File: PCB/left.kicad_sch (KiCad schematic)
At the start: 3 parts, among them J1 AudioJack4, U1 MOUDLE-SEEEDUINO-XIAO, U2 MCP23017_ML

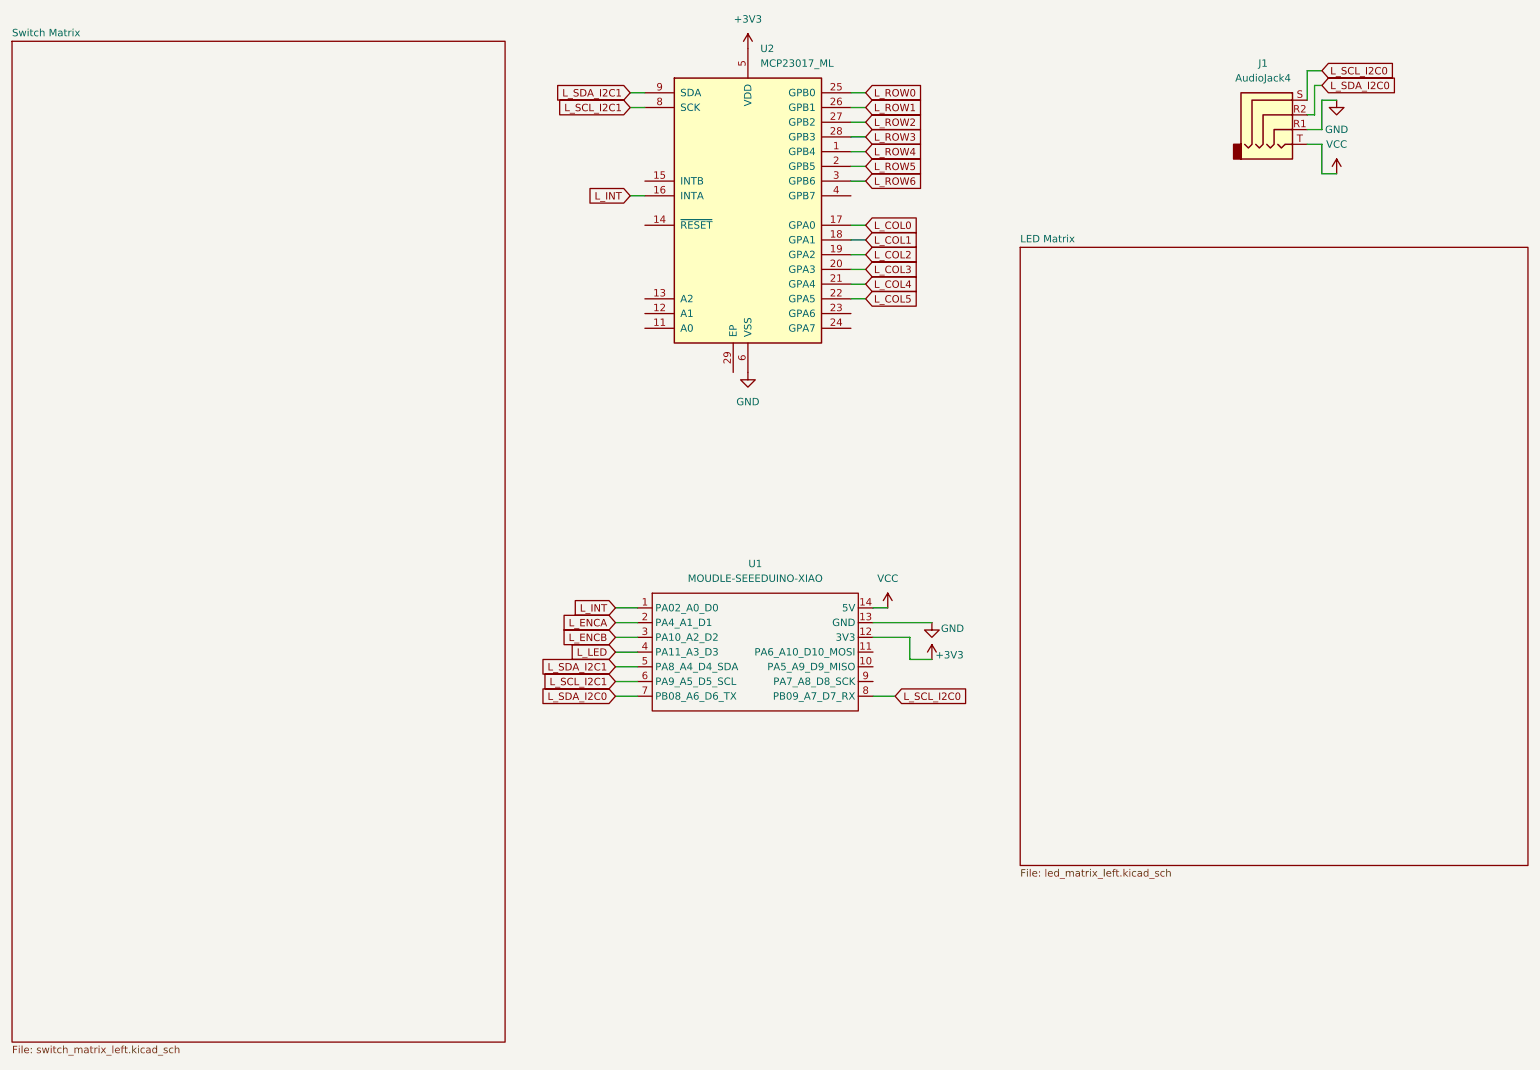
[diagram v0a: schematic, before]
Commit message: updated schematic
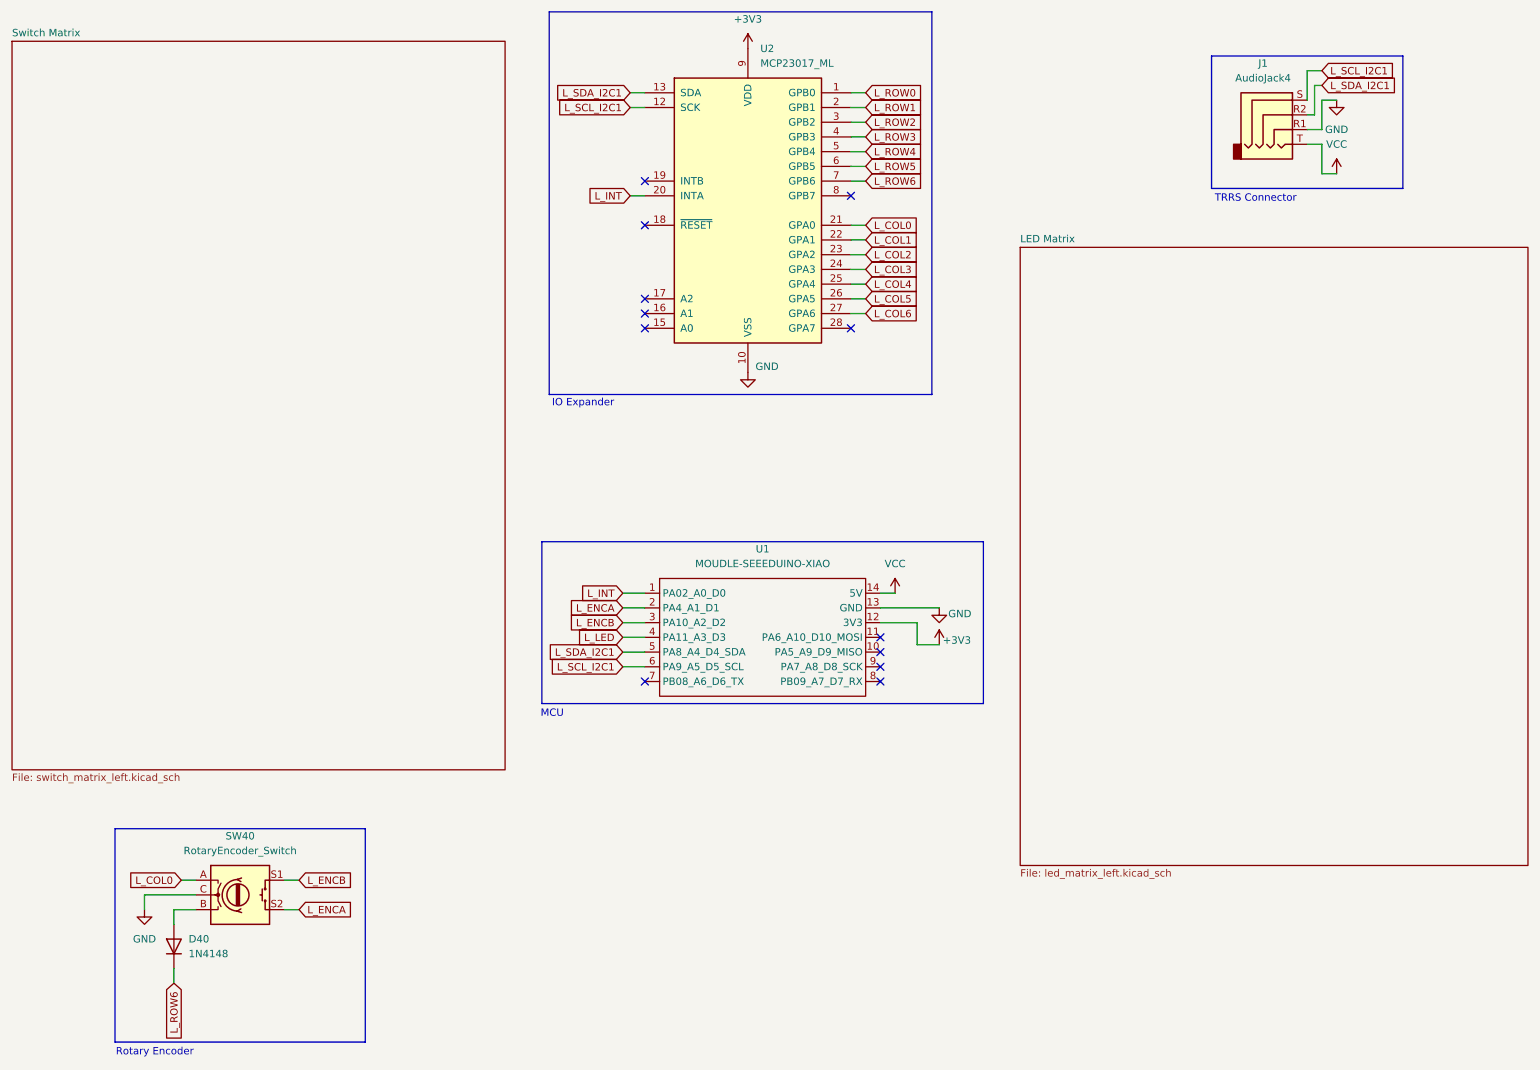
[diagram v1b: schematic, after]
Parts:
- added D40: 1N4148, Diode_THT:D_DO-35_SOD27_P7.62mm_Horizontal, symbol Diode:1N4148
- added SW40: RotaryEncoder_Switch, symbol Device:RotaryEncoder_Switch
- U2: symbol Interface_Expansion:MCP23017_ML -> Interface_Expansion:MCP23017_SP
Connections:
- net +3V3: now also U2.9 (VDD); no longer U2.5 (VDD)
- net GND: now also U2.10 (VSS), SW40.C; no longer U2.6 (VSS)
- net L_COL0: now also U2.21 (GPA0), SW40.A; no longer U2.17 (GPA0)
- net L_COL1: now also U2.22 (GPA1); no longer U2.18 (GPA1)
- net L_COL2: now also U2.23 (GPA2); no longer U2.19 (GPA2)
- net L_COL3: now also U2.24 (GPA3); no longer U2.20 (GPA3)
- net L_COL4: now also U2.25 (GPA4); no longer U2.21 (GPA4)
- net L_COL5: now also U2.26 (GPA5); no longer U2.22 (GPA5)
- net L_ENCA: now also SW40.S2
- net L_ENCB: now also SW40.S1
- net L_INT: now also U2.20 (INTA); no longer U2.16 (INTA)
- net L_ROW0: now also U2.1 (GPB0); no longer U2.25 (GPB0)
- net L_ROW1: now also U2.2 (GPB1); no longer U2.26 (GPB1)
- net L_ROW2: now also U2.3 (GPB2); no longer U2.27 (GPB2)
- net L_ROW3: now also U2.4 (GPB3); no longer U2.28 (GPB3)
- net L_ROW4: now also U2.5 (GPB4); no longer U2.1 (GPB4)
- net L_ROW5: now also U2.6 (GPB5); no longer U2.2 (GPB5)
- net L_ROW6: now also U2.7 (GPB6), D40.1 (K); no longer U2.3 (GPB6)
- net L_SCL_I2C1: now also J1.S, U2.12 (SCK); no longer U2.8 (SCK)
- net L_SDA_I2C1: now also J1.R2, U2.13 (SDA); no longer U2.9 (SDA)
- net L_SCL_I2C0: no longer names the net of U1.8 (PB09_A7_D7_RX)
- net L_SCL_I2C0: no longer J1.S
- net L_SDA_I2C0: no longer names the net of U1.7 (PB08_A6_D6_TX)
- net L_SDA_I2C0: no longer J1.R2
- new net: D40.2 (A), SW40.B
- new net L_COL6: U2.27 (GPA6)
- no-connect marks 0 -> 12
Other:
- note added: "IO Expander"
- note added: "MCU"
- note added: "Rotary Encoder"
- note added: "TRRS Connector"
- moved on the sheet: U1

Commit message: routed the switches and diodes
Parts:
- SW40: footprint (none) -> Rotary_Encoder:RotaryEncoder_Alps_EC11E-Switch_Vertical_H20mm
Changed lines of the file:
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@@
 			)
 		)
-		(property "Footprint" ""
+		(property "Footprint" "Rotary_Encoder:RotaryEncoder_Alps_EC11E-Switch_Vertical_H20mm"
 			(at 54.61 162.306 0)
 			(effects
